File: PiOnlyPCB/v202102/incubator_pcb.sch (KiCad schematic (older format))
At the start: 34 parts, among them J1 Conn_01x04, J10 Conn_01x02, J11 Conn_01x02, J2 Conn_01x04, J3 Conn_01x04, J4 Conn_01x02, J5 Conn_01x02, J6 Conn_01x02, J7 Conn_01x02, J8 Conn_01x02, J9 Conn_01x02, Q1 Q_NMOS_GDS, Q2 Q_NMOS_GDS, Q3 Q_NMOS_GDS, Q4 Q_NMOS_GDS, U1 header_pi_zero_w

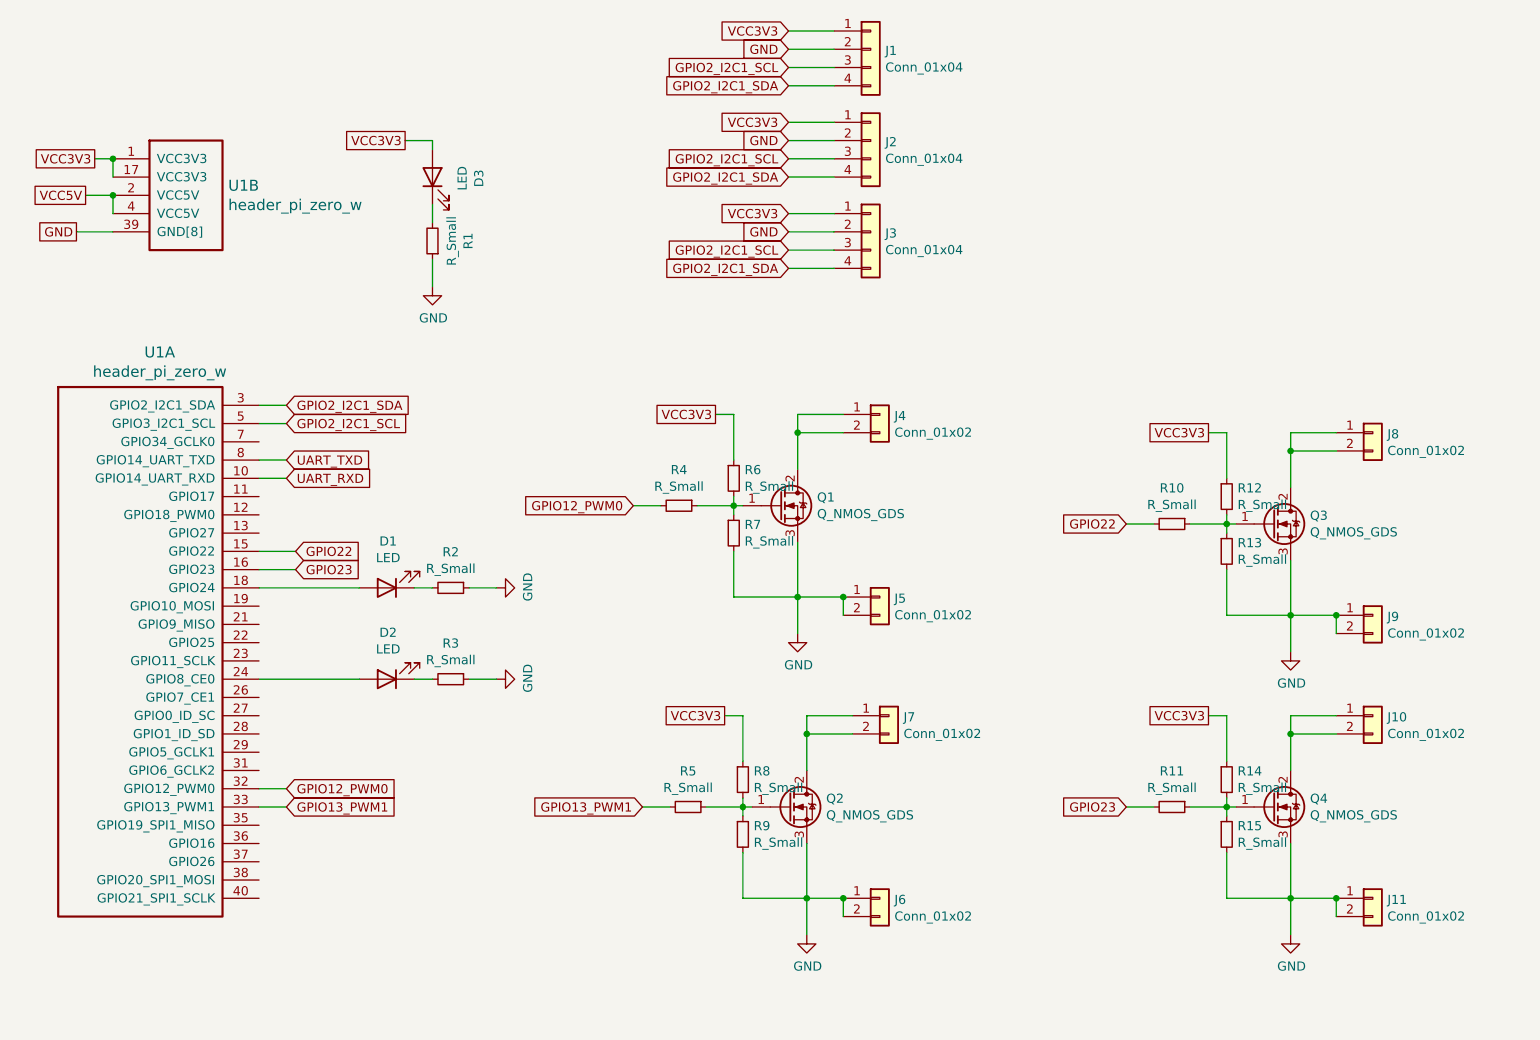
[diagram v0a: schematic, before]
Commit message: Partial version with GPIO expander too.
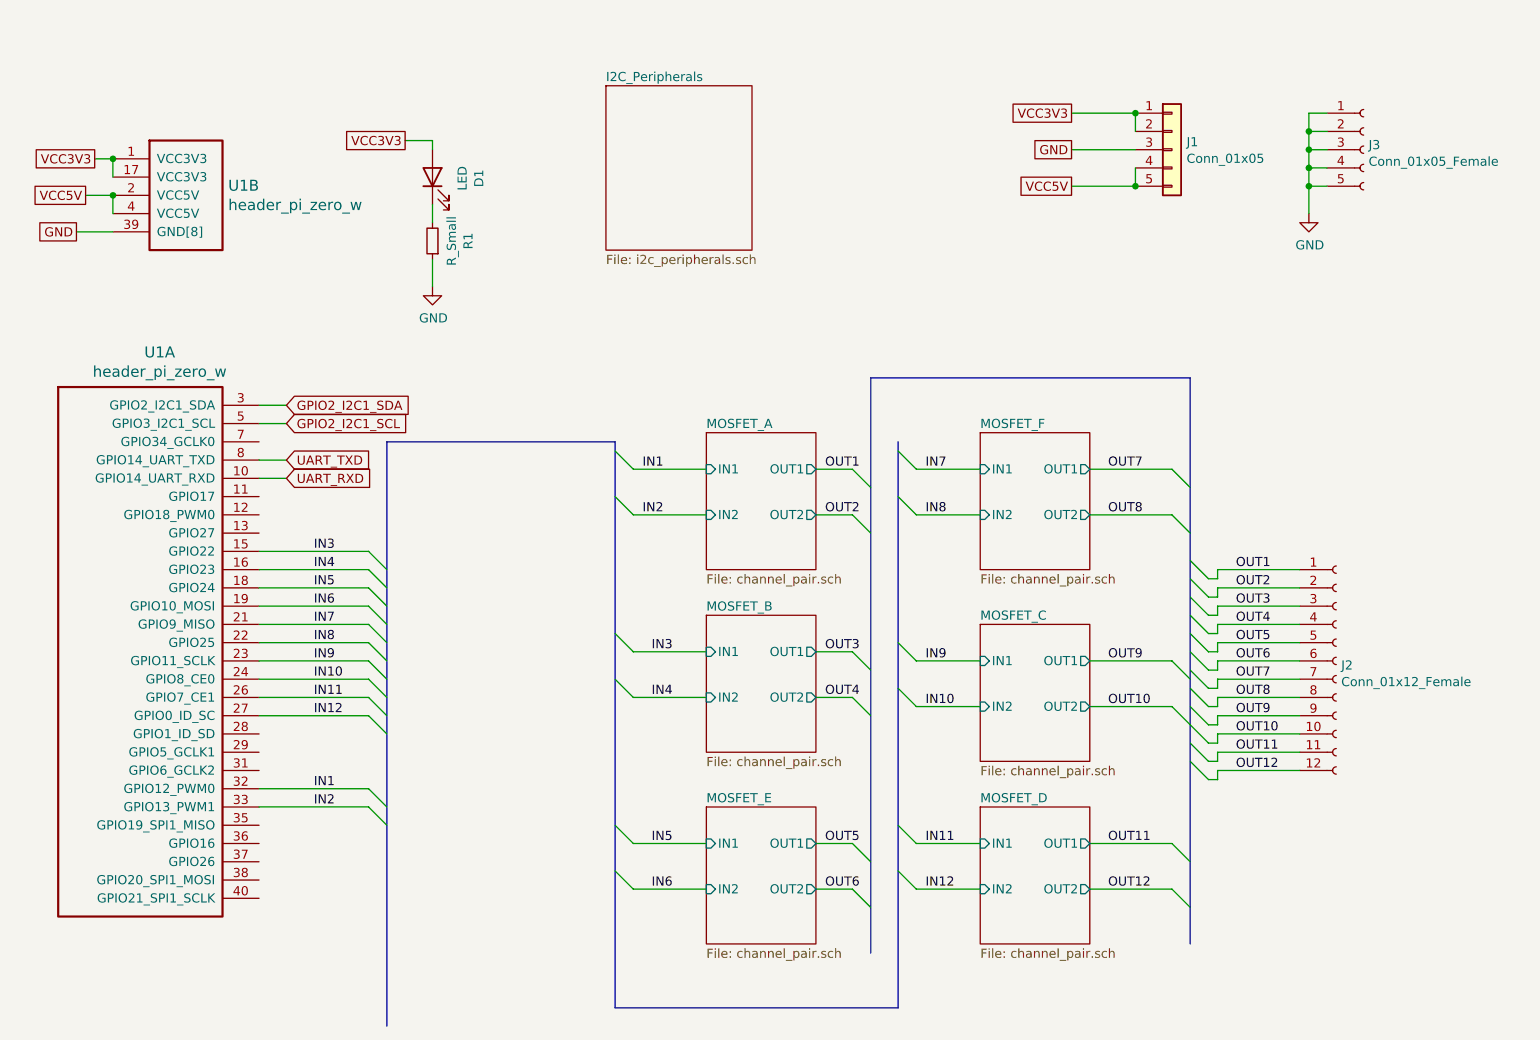
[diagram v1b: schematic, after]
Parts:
- removed D1, D2: LED, Diode_SMD:D_0805_2012Metric_Pad1.15x1.40mm_HandSolder, symbol Device:LED
- removed J1, J2, J3: Conn_01x04, Connector_PinHeader_2.54mm:PinHeader_1x04_P2.54mm_Vertical, symbol Connector_Generic:Conn_01x04
- removed J10, J11, J4, J5, J6, J7, J8, J9: Conn_01x02, TerminalBlock_Phoenix:TerminalBlock_Phoenix_MKDS-1,5-2_1x02_P5.00mm_Horizontal, symbol Connector_Generic:Conn_01x02
- removed Q1, Q2, Q3, Q4: Q_NMOS_GDS, Package_TO_SOT_THT:TO-220-3_Vertical, symbol Device:Q_NMOS_GDS
- removed R10, R11, R12, R13, R14, R15, R2, R3, R4, R5, R6, R7, R8, R9: R_Small, Resistor_SMD:R_0805_2012Metric_Pad1.15x1.40mm_HandSolder, symbol Device:R_Small
- added J1: Conn_01x05, Connector_PinHeader_2.54mm:PinHeader_1x05_P2.54mm_Vertical, symbol Connector_Generic:Conn_01x05
- added J2: Conn_01x12_Female, v202102_OpenPlant:PWRCON_3M81-12, symbol Connector:Conn_01x12_Female
- added J3: Conn_01x05_Female, v202102_OpenPlant:PWRCON_3M81-5, symbol Connector:Conn_01x05_Female
- R1: footprint Resistor_SMD:R_0805_2012Metric_Pad1.15x1.40mm_HandSolder -> Resistor_SMD:R_0805_2012Metric_Pad1.20x1.40mm_HandSolder
- renumbered D3 to D1
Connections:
- net GND: now also J1.3 (Pin_3), J3.1 (Pin_1), J3.2 (Pin_2), J3.3 (Pin_3), J3.4 (Pin_4), J3.5 (Pin_5)
- net VCC3V3: now also J1.1 (Pin_1), J1.2 (Pin_2)
- net VCC5V: now also J1.4 (Pin_4), J1.5 (Pin_5)
- net IN5: now reaches U1.18 (GPIO24)
- net IN6: now reaches U1.19 (GPIO10_MOSI)
- net IN7: now reaches U1.21 (GPIO9_MISO)
- net IN8: now reaches U1.22 (GPIO25)
- net IN9: now reaches U1.23 (GPIO11_SCLK)
- net IN10: now reaches U1.24 (GPIO8_CE0)
- net IN11: now reaches U1.26 (GPIO7_CE1)
- net IN12: now reaches U1.27 (GPIO0_ID_SC)
- net GPIO12_PWM0 renamed IN1
- net GPIO13_PWM1 renamed IN2
- net GPIO22 renamed IN3
- net GPIO23 renamed IN4
- new net OUT1: J2.1 (Pin_1)
- new net OUT10: J2.10 (Pin_10)
- new net OUT11: J2.11 (Pin_11)
- new net OUT12: J2.12 (Pin_12)
- new net OUT2: J2.2 (Pin_2)
- new net OUT3: J2.3 (Pin_3)
- new net OUT4: J2.4 (Pin_4)
- new net OUT5: J2.5 (Pin_5)
- new net OUT6: J2.6 (Pin_6)
- new net OUT7: J2.7 (Pin_7)
- new net OUT8: J2.8 (Pin_8)
- new net OUT9: J2.9 (Pin_9)
